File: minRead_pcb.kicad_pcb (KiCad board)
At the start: 2 copper layers, 151.5 x 148.6 mm, 119 parts, among them J1 USB_C_Receptacle, J2 FH34SRJ-24S-0.5SH_50_, J3 FH34SRJ-6S-0.5SH_50_, J5 Conn_01x02, J7 Micro_SD_Card, Q10 BSS138, Q11 BSS138, Q16 MMBT3906, Q17 MMBT3904, Q18 AO3419, Q4 [BSS138] AO3400A, Q5 AO3419, Q6 AO3419, SW1 SW_Push, SW10 SW_Push, SW11 SW_Push, SW2 SW_Push, SW3 SW_Push, SW4 SW_Push, SW6 SW_Push, SW8 SW_Push, SW9 SW_Push, U1 TPD4E1U06DBVR, U11 AP3031KTR, U3 AP2112K-3.3, U4 ESP32-S3-WROOM-1, U6 TPD4E1U06DBVR, U7 MCP73832-2-OT

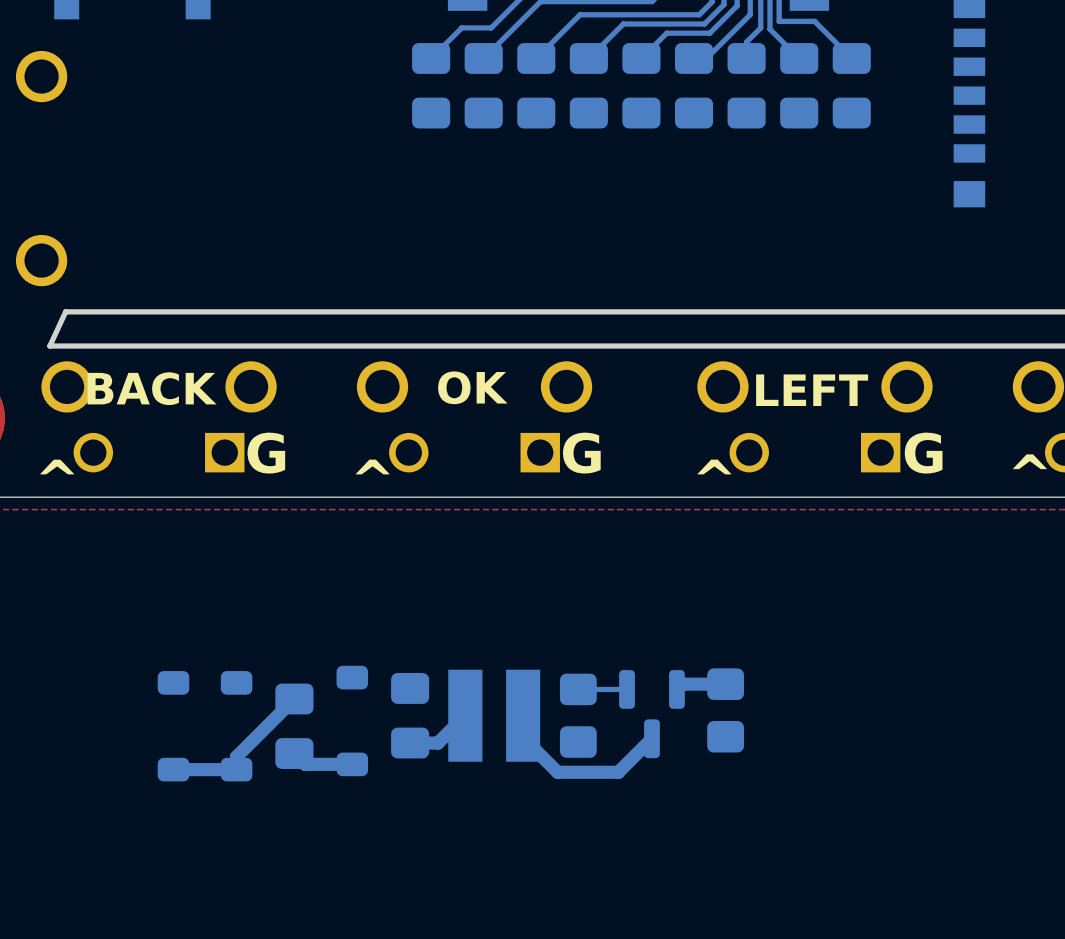
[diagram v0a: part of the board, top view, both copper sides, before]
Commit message: charge pump in place
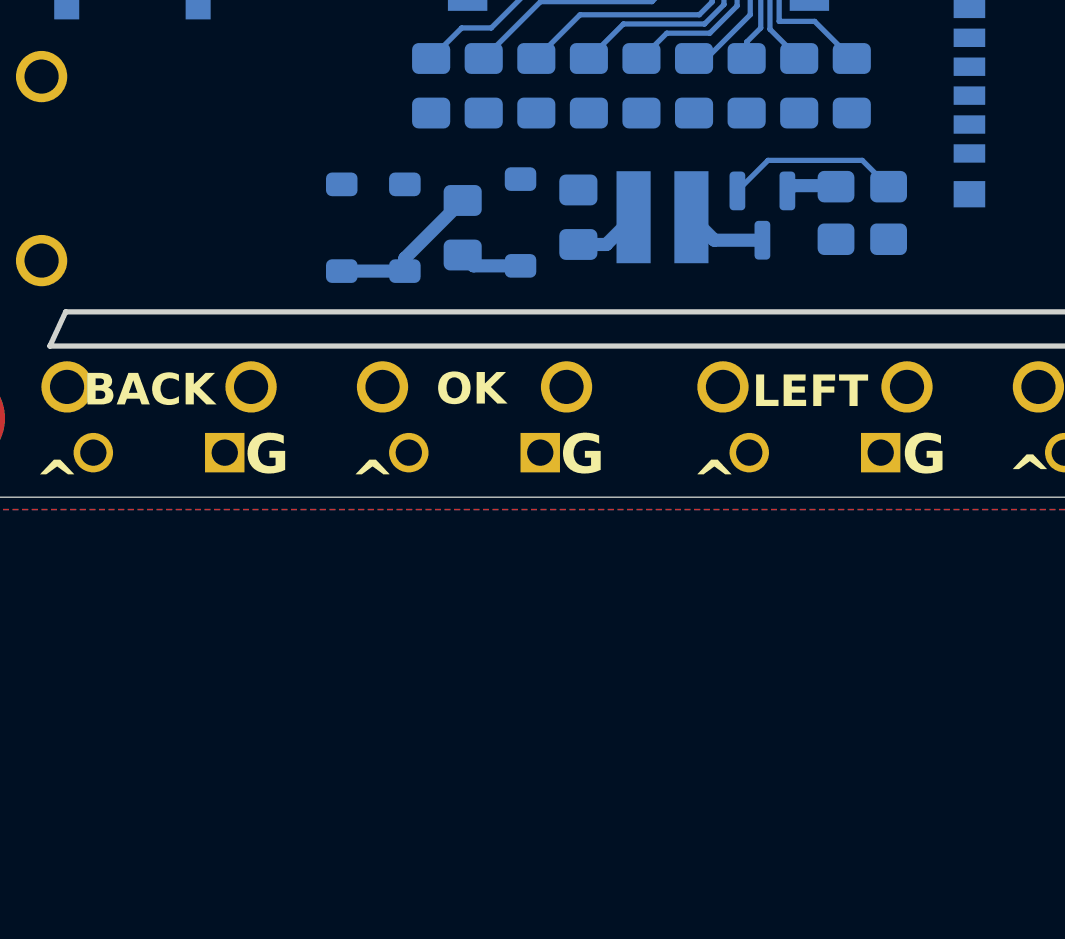
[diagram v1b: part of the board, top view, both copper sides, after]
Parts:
- moved R15 22.5 mm to (83.0, 137.4)
- moved C10 20.0 mm to (71.2, 137.6)
- moved D6 20.0 mm to (62.2, 138.0)
- moved L1 20.0 mm to (74.4, 137.6)
- moved C11 20.0 mm to (66.8, 138.0)
- moved D4 20.0 mm to (64.6, 138.0)
- moved D5 20.0 mm to (69.0, 137.8)
- moved Q4 19.4 mm to (78.2, 137.5)
- moved R14 19.4 mm to (81.0, 137.4)
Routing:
- net /GDR: track 1.85 -> 6.65 mm
- net Net-(D5-A): track 9.18 -> 5.43 mm
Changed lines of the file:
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@@
 	(footprint "Capacitor_SMD:C_0805_2012Metric_Pad1.18x1.45mm_HandSolder"
 		(layer "B.Cu")
-		(at 64.8 156.5625 -90)
+		(at 71.2 137.6 -90)
 		(descr "Capacitor SMD 0805 (2012 Metric), square (rectangular) end terminal, IPC-7351 nominal with elongated pad for handsoldering. (Body size source: IPC-SM-782 page 76, https://www.pcb-3d.com/wordpress/wp-content/uploads/ipc-sm-782a_amendment_1_and_2.pdf, https://docs.google.com/spreadsheets/d/1BsfQQcO9C6DZCsRaXUlFlo91Tg2WpOkGARC1WS5S8t0/edit?usp=sharing), generated with kicad-footprint-generator")
 		(tags "capacitor handsolder")
@@
 	(footprint "Capacitor_SMD:C_0805_2012Metric_Pad1.18x1.45mm_HandSolder"
 		(layer "B.Cu")
-		(at 60.4 156.9625 -90)
+		(at 66.8 138 -90)
 		(descr "Capacitor SMD 0805 (2012 Metric), square (rectangular) end terminal, IPC-7351 nominal with elongated pad for handsoldering. (Body size source: IPC-SM-782 page 76, https://www.pcb-3d.com/wordpress/wp-content/uploads/ipc-sm-782a_amendment_1_and_2.pdf, https://docs.google.com/spreadsheets/d/1BsfQQcO9C6DZCsRaXUlFlo91Tg2WpOkGARC1WS5S8t0/edit?usp=sharing), generated with kicad-footprint-generator")
 		(tags "capacitor handsolder")
@@
 	(footprint "Package_TO_SOT_SMD:SOT-23"
 		(layer "B.Cu")
-		(at 74 156.5 -90)
+		(at 78.2 137.5375 -90)
 		(descr "SOT, 3 Pin (JEDEC TO-236 Var AB https://www.jedec.org/document_search?search_api_views_fulltext=TO-236), generated with kicad-footprint-generator ipc_gullwing_generator.py")
 		(tags "SOT TO_SOT_SMD")
@@
 	(footprint "Resistor_SMD:R_0805_2012Metric_Pad1.20x1.40mm_HandSolder"
 		(layer "B.Cu")
-		(at 71.2 156.5625 90)
+		(at 83 137.4375 90)
 		(descr "Resistor SMD 0805 (2012 Metric), square (rectangular) end terminal, IPC-7351 nominal with elongated pad for handsoldering. (Body size source: IPC-SM-782 page 72, https://www.pcb-3d.com/wordpress/wp-content/uploads/ipc-sm-782a_amendment_1_and_2.pdf), generated with kicad-footprint-generator")
 		(tags "resistor handsolder")
@@
 	(footprint "Diode_SMD:D_SOD-123"
 		(layer "B.Cu")
-		(at 55.8 156.9625 -90)
+		(at 62.2 138 -90)
 		(descr "SOD-123")
 		(tags "SOD-123")
@@
 	(footprint "Diode_SMD:D_SOD-123"
 		(layer "B.Cu")
-		(at 62.6 156.7625 -90)
+		(at 69 137.8 -90)
 		(descr "SOD-123")
 		(tags "SOD-123")
@@
 	(footprint "Resistor_SMD:R_0805_2012Metric_Pad1.20x1.40mm_HandSolder"
 		(layer "B.Cu")
-		(at 76.8 156.3625 90)
+		(at 81 137.4375 90)
 		(descr "Resistor SMD 0805 (2012 Metric), square (rectangular) end terminal, IPC-7351 nominal with elongated pad for handsoldering. (Body size source: IPC-SM-782 page 72, https://www.pcb-3d.com/wordpress/wp-content/uploads/ipc-sm-782a_amendment_1_and_2.pdf), generated with kicad-footprint-generator")
 		(tags "resistor handsolder")
@@
 	(footprint "Diode_SMD:D_SOD-123"
 		(layer "B.Cu")
-		(at 58.2 156.9625 90)
+		(at 64.6 138 90)
 		(descr "SOD-123")
 		(tags "SOD-123")
@@
 	(footprint "srn3010C-100m:IND_SRN3010C-100M"
 		(layer "B.Cu")
-		(at 68 156.5625 180)
+		(at 74.4 137.6 180)
 		(property "Reference" "L1"
 			(at 0 2.25 0)
@@
 	)
 	(segment
-		(start 64.8 157.6)
-		(end 65.8625 157.6)
+		(start 71.2 138.6375)
+		(end 72.2625 138.6375)
 		(width 0.5)
 		(layer "B.Cu")
@@
 	)
 	(segment
-		(start 65.8625 157.6)
-		(end 66.9 156.5625)
+		(start 72.2625 138.6375)
+		(end 73.3 137.6)
 		(width 0.5)
 		(layer "B.Cu")
@@
 	)
 	(segment
-		(start 60.4 155.925)
-		(end 58.2 158.125)
+		(start 66.8 136.9625)
+		(end 64.6 139.1625)
 		(width 0.5)
 		(layer "B.Cu")
@@
 	)
 	(segment
-		(start 58.2 158.125)
-		(end 58.2 158.6125)
+		(start 64.6 139.1625)
+		(end 64.6 139.65)
 		(width 0.5)
 		(layer "B.Cu")
@@
 	)
 	(segment
-		(start 55.8 158.6125)
-		(end 58.2 158.6125)
+		(start 62.2 139.65)
+		(end 64.6 139.65)
 		(width 0.5)
 		(layer "B.Cu")
@@
 	)
 	(segment
-		(start 62.6 158.4125)
-		(end 60.8125 158.4125)
+		(start 69 139.45)
+		(end 67.2125 139.45)
 		(width 0.5)
 		(layer "B.Cu")
@@
 	)
 	(segment
-		(start 60.8125 158.4125)
-		(end 60.4 158)
+		(start 67.2125 139.45)
+		(end 66.8 139.0375)
 		(width 0.5)
 		(layer "B.Cu")
@@
 	)
 	(segment
-		(start 69.1 157.400798)
-		(end 69.1 156.5625)
+		(start 76.375 138.475)
+		(end 78.2 138.475)
 		(width 0.5)
 		(layer "B.Cu")
@@
 	)
 	(segment
-		(start 72.725 158.7125)
-		(end 70.411702 158.7125)
-		(width 0.5)
-		(layer "B.Cu")
-		(net "Net-(D5-A)")
-	)
-	(segment
-		(start 70.411702 158.7125)
-		(end 69.1 157.400798)
-		(width 0.5)
-		(layer "B.Cu")
-		(net "Net-(D5-A)")
-	)
-	(segment
-		(start 74 157.4375)
-		(end 72.725 158.7125)
+		(start 75.5 137.6)
+		(end 76.375 138.475)
 		(width 0.5)
 		(layer "B.Cu")
@@
 	)
 	(segment
-		(start 73.05 155.5625)
-		(end 71.2 155.5625)
+		(start 78.4125 135.4375)
+		(end 77.25 136.6)
+		(width 0.2)
+		(layer "B.Cu")
+		(net "/GDR")
+	)
+	(segment
+		(start 83 136.4375)
+		(end 82 135.4375)
+		(width 0.2)
+		(layer "B.Cu")
+		(net "/GDR")
+	)
+	(segment
+		(start 82 135.4375)
+		(end 78.4125 135.4375)
 		(width 0.2)
 		(layer "B.Cu")
@@
 	)
 	(segment
-		(start 76.8 155.3625)
-		(end 75.15 155.3625)
+		(start 81 136.4)
+		(end 79.35 136.4)
 		(width 0.5)
 		(layer "B.Cu")
@@
 	)
 	(segment
-		(start 75.15 155.3625)
-		(end 74.95 155.5625)
+		(start 79.35 136.4)
+		(end 79.15 136.6)
 		(width 0.5)
 		(layer "B.Cu")
